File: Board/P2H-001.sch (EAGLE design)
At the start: 28 parts, among them IC1 74LS157N, IC2 LTC485N, IC3 4051N, IC4 74LS07N, IC5 LTC485N

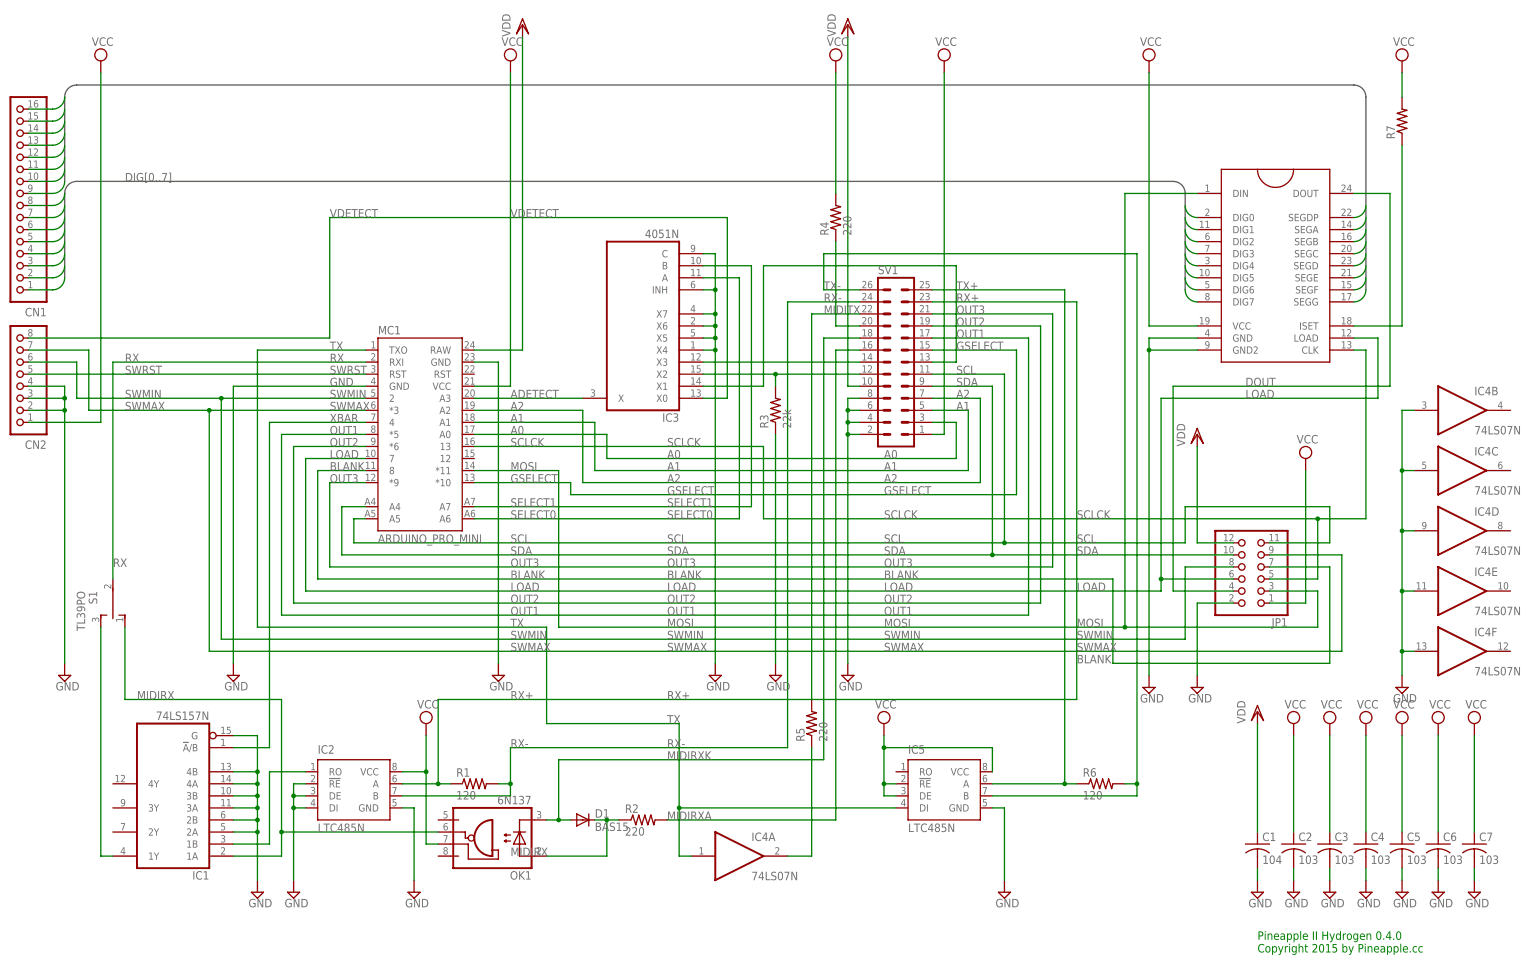
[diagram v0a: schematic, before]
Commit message: Refine of sch.
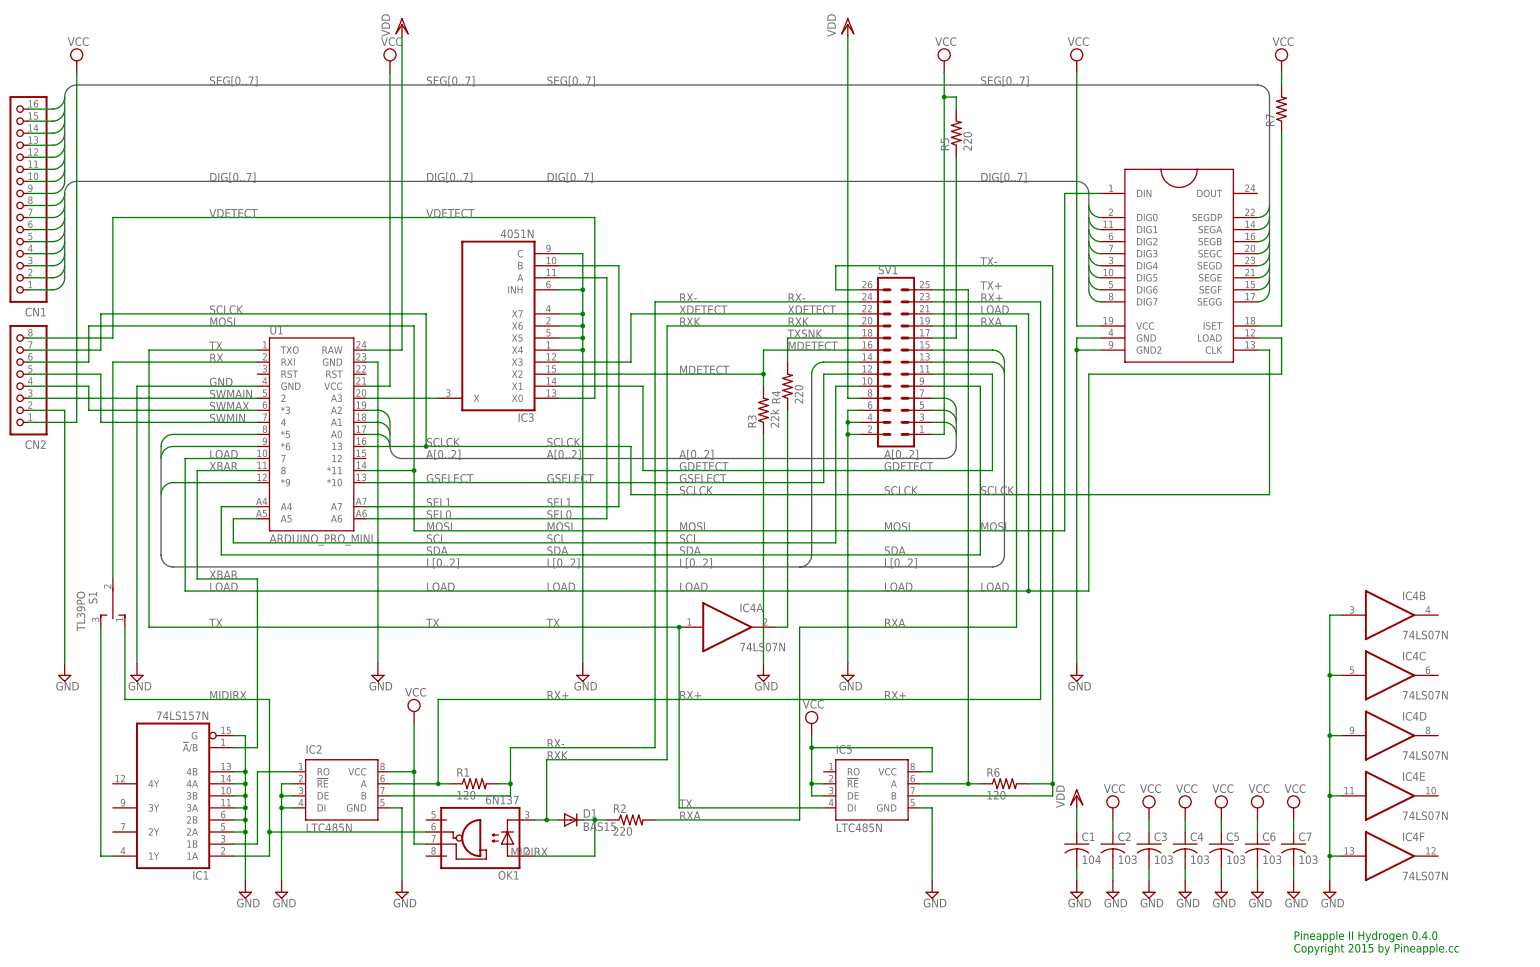
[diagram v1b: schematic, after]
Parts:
- removed JP1: (no value), pinhead:PINHD-2X6
- removed MC1: ARDUINO_PRO_MINI, SparkFun-Boards:ARDUINO_PRO_MINI
- removed MC2: MAX7219DIP, SparkFun-DigitalIC:MAX7219DIP
- added U1: ARDUINO_PRO_MINI, SparkFun-Boards:ARDUINO_PRO_MINI
- added U2: MAX7219DIP, SparkFun-DigitalIC:MAX7219DIP
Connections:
- removed net BLANK: JP1.7, MC1.8
- removed net DOUT: JP1.4, MC2.DOUT
- removed net MIDIRXA: R2.2, SV1.16
- removed net MIDIRXK: D1.A, OK1.C, SV1.18
- removed net MIDITX: R5.2, SV1.22
- removed net N$3: IC3A.X1, SV1.13
- removed net N$5: IC3A.X2, R3.2, SV1.12
- removed net N$6: IC3A.X3, SV1.14
- removed net OUT1: MC1.*5, SV1.17
- removed net OUT2: MC1.*6, SV1.19
- removed net OUT3: MC1.*9, SV1.21
- removed net SELECT0: IC3A.A, MC1.A6
- removed net SELECT1: IC3A.B, MC1.A7
- removed net SWRST: CN2.5, MC1.RST
- new net GDETECT: IC3A.X1, SV1.11
- new net L0: SV1.13, U1.*5
- new net L1: SV1.14, U1.*6
- new net L2: SV1.15, U1.*9
- new net MDETECT: IC3A.X2, R3.2, SV1.16
- new net RXA: R2.2, SV1.19
- new net RXK: D1.A, OK1.C, SV1.20
- new net SEL0: IC3A.A, U1.A6
- new net SEL1: IC3A.B, U1.A7
- new net SWMAIN: CN2.3, U1.2
- new net TXSNK: R4.2, SV1.18
- new net XDETECT: IC3A.X3, SV1.22
- net A0: now also U1.A0; no longer MC1.A0
- net A1: now also U1.A1; no longer MC1.A1
- net A2: now also U1.A2; no longer MC1.A2
- net ADETECT: now also U1.A3; no longer MC1.A3
- net DIG0: now also U2.DIG0; no longer MC2.DIG0
- net DIG1: now also U2.DIG1; no longer MC2.DIG1
- net DIG2: now also U2.DIG2; no longer MC2.DIG2
- net DIG3: now also U2.DIG3; no longer MC2.DIG3
- net DIG4: now also U2.DIG4; no longer MC2.DIG4
- net DIG5: now also U2.DIG5; no longer MC2.DIG5
- net DIG6: now also U2.DIG6; no longer MC2.DIG6
- net DIG7: now also U2.DIG7; no longer MC2.DIG7
- net GND: now also U1.GND, U1.GND@2, U2.GND, U2.GND2; no longer CN2.3, CN2.4, JP1.2, MC1.GND, MC1.GND@2, MC2.GND, MC2.GND2, SV1.8
- net GSELECT: now also SV1.12, U1.*10; no longer MC1.*10, SV1.15
- net LOAD: now also SV1.21, U1.7, U2.LOAD; no longer JP1.6, MC1.7, MC2.LOAD
- net MOSI: now also CN2.6, U1.*11, U2.DIN; no longer JP1.3, MC1.*11, MC2.DIN
- net N$12: now also R5.1, SV1.17; no longer R4.1, SV1.20
- net N$2: now also R4.1; no longer R5.1
- net N$21: now also U2.ISET; no longer MC2.ISET
- net RX: now also U1.RXI; no longer MC1.RXI
- net SCL: now also SV1.10, U1.A5; no longer JP1.11, MC1.A5, SV1.11
- net SCLCK: now also CN2.7, U1.13, U2.CLK; no longer JP1.5, MC1.13, MC2.CLK
- net SDA: now also U1.A4; no longer JP1.10, MC1.A4
- net SEG0: now also U2.SEGG; no longer MC2.SEGG
- net SEG1: now also U2.SEGF; no longer MC2.SEGF
- net SEG2: now also U2.SEGE; no longer MC2.SEGE
- net SEG3: now also U2.SEGD; no longer MC2.SEGD
- net SEG4: now also U2.SEGC; no longer MC2.SEGC
- net SEG5: now also U2.SEGB; no longer MC2.SEGB
- net SEG6: now also U2.SEGA; no longer MC2.SEGA
- net SEG7: now also U2.SEGDP; no longer MC2.SEGDP
- net SWMAX: now also CN2.4, U1.*3; no longer CN2.7, JP1.9, MC1.*3
- net SWMIN: now also CN2.5, U1.4; no longer CN2.6, JP1.8, MC1.2
- net TX: now also U1.TXO; no longer MC1.TXO
- net VCC: now also R5.2, U1.VCC, U2.VCC; no longer JP1.1, MC1.VCC, MC2.VCC, R4.2
- net VDD: now also SV1.8, U1.RAW; no longer JP1.12, MC1.RAW, SV1.10
- net XBAR: now also U1.8; no longer MC1.4
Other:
- moved on the sheet: C1, C2, C3, C4, C5, C6, C7, D1, IC2, IC3, IC4A, IC4B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
